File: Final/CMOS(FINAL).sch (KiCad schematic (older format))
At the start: 1 part, among them U9 28F010

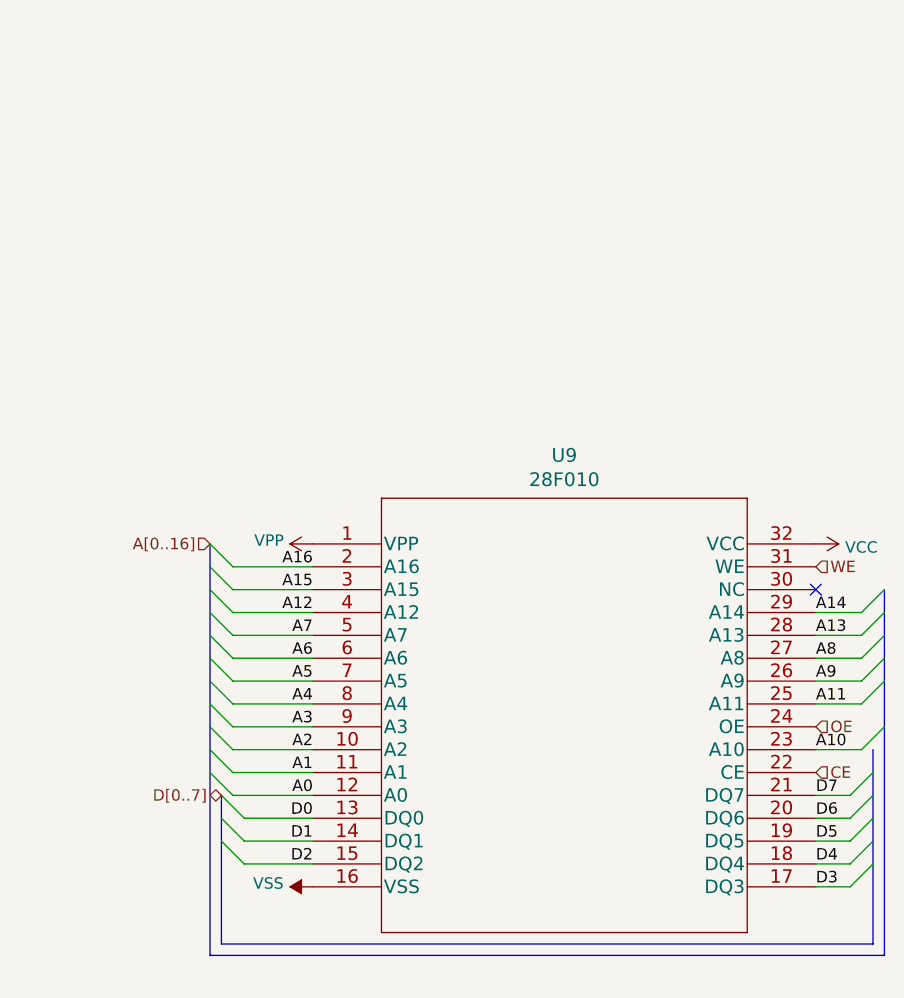
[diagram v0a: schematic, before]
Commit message: For Commenting
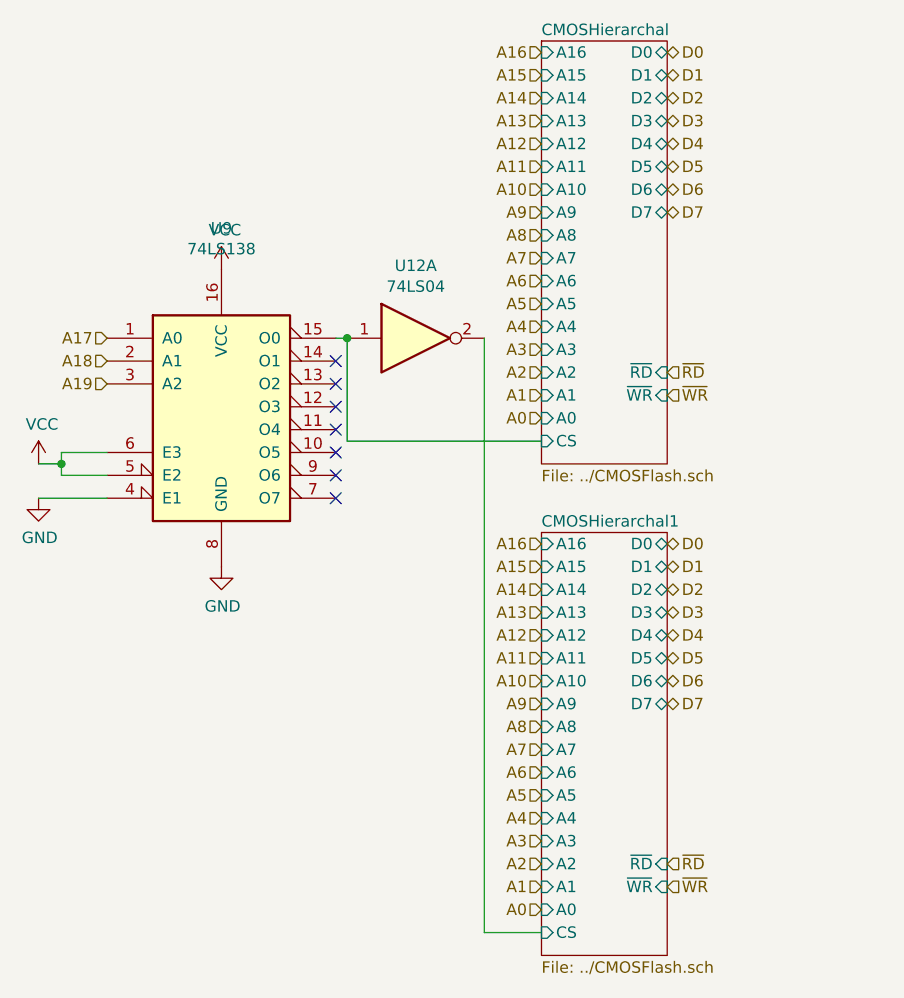
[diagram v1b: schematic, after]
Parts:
- removed U9: 28F010, 28F010, symbol 28F010:28F010
- added U12: 74LS04, symbol 74xx:74LS04
- added U9: 74LS138, symbol 74xx:74LS138
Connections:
- net VCC: now also U9.16 (VCC), U9.5 (E2), U9.6 (E3)
- new net A17: U9.1 (A0)
- new net A18: U9.2 (A1)
- new net A19: U9.3 (A2)
- new net CMOSHierarchal/CS: U12.1, U9.15 (O0)
- new net CMOSHierarchal1/CS: U12.2
- new net GND: U9.4 (E1), U9.8 (GND)
- no-connect marks 1 -> 7

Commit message: Hopefully the board is here
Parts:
- U12: footprint (none) -> Package_DIP:DIP-14_W7.62mm
- U9: footprint (none) -> Package_DIP:DIP-16_W7.62mm
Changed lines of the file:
@@
 F 0 "U9" H 3950 3681 50  0000 C CNN
 F 1 "74LS138" H 3950 3590 50  0000 C CNN
-F 2 "" H 3950 2900 50  0001 C CNN
+F 2 "Package_DIP:DIP-16_W7.62mm" H 3950 2900 50  0001 C CNN
 F 3 "http://www.ti.com/lit/gpn/sn74LS138" H 3950 2900 50  0001 C CNN
 	1    3950 2900
@@
 F 0 "U12" H 4800 2917 50  0000 C CNN
 F 1 "74LS04" H 4800 2826 50  0000 C CNN
-F 2 "" H 4800 2600 50  0001 C CNN
+F 2 "Package_DIP:DIP-14_W7.62mm" H 4800 2600 50  0001 C CNN
 F 3 "http://www.ti.com/lit/gpn/sn74LS04" H 4800 2600 50  0001 C CNN
 	1    4800 2600
